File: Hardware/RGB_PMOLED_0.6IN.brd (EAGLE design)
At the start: 160 x 100 mm, 25 parts, among them Q1 310mA/60V/1.6Ω, U1 UG-6464TDDBG01-EXT, U2 AP3012, U3 3.3V, U4 TXB0104

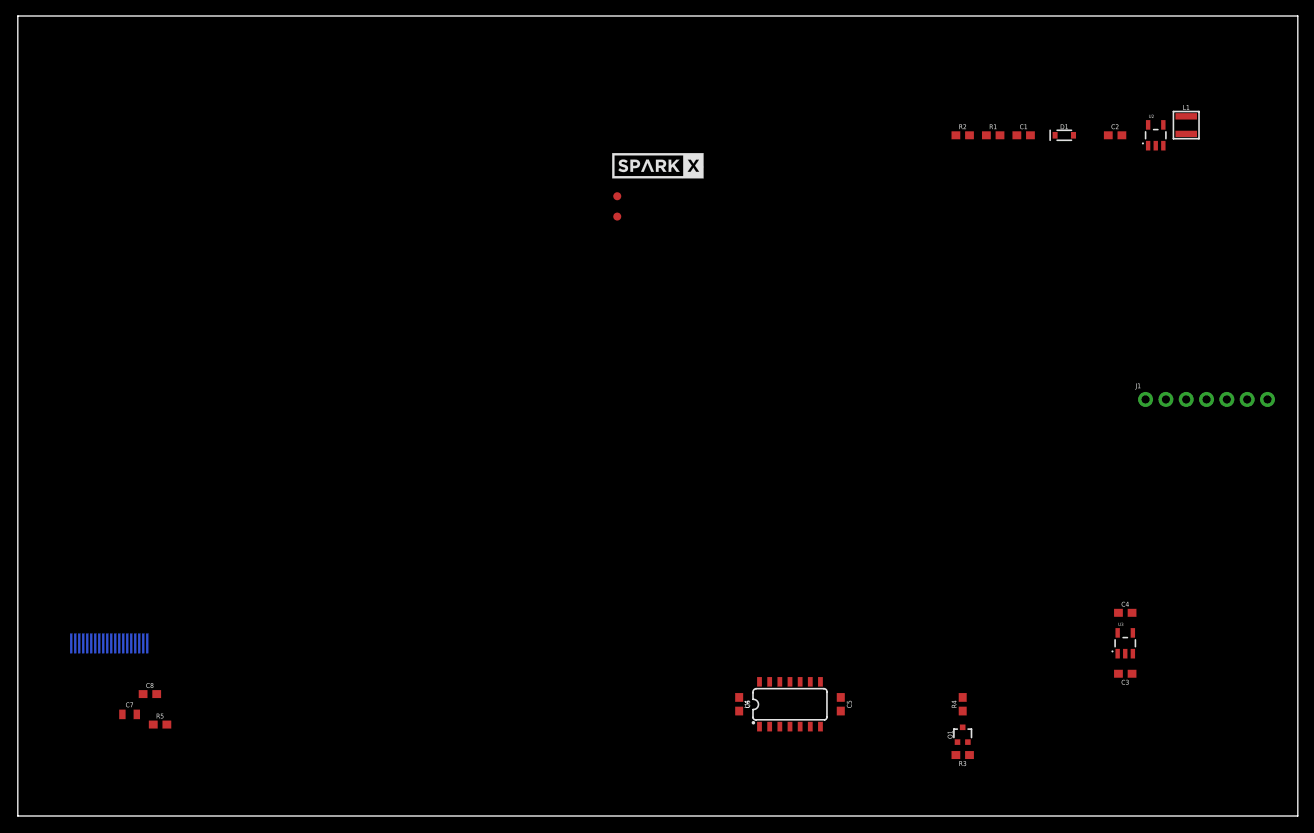
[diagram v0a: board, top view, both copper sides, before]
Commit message: First revision
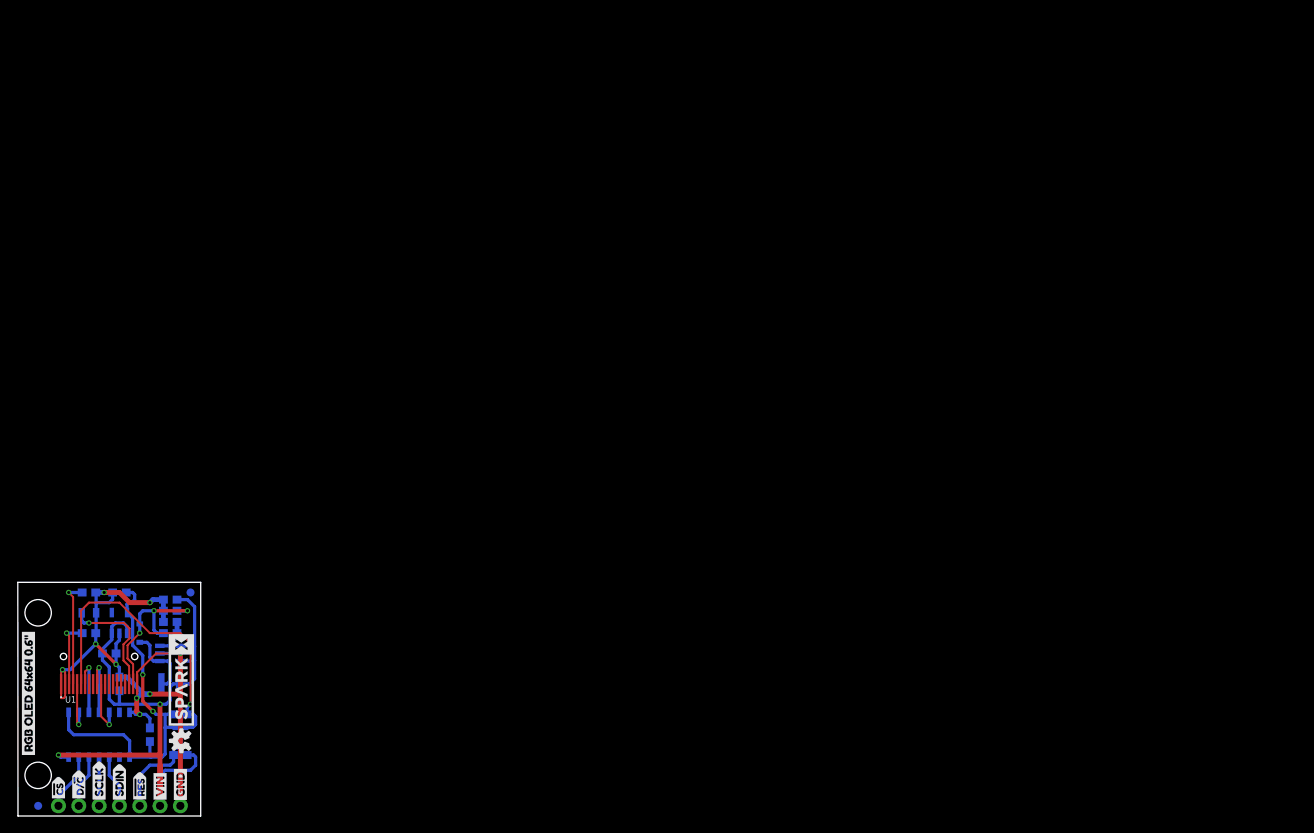
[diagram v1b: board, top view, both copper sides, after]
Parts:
- added H1, H2: STAND-OFF, SparkFun-Hardware:STAND-OFF
- added LOGO2, LOGO4: OSHW-LOGOS, SparkFun-Aesthetics:OSHW-LOGO-S
- added LOGO3: SPARKX-LOGO5, 1.81_Greyscale_OLED_Breakout:SPARKX-LARGE
- added U$1, U$2: (no value), buzzard_labels:VIN0
- added U$10, U$11: (no value), buzzard_labels:#RES2
- added U$12, U$13: (no value), buzzard_labels:#CS6
- added U$14, U$9: (no value), buzzard_labels:D##C5
- added U$16: (no value), buzzard_labels:RGB_OLED_64X64_0#6#7
- added U$3, U$4: (no value), buzzard_labels:SDIN3
- added U$5, U$6: (no value), buzzard_labels:SCLK4
- added U$7, U$8: (no value), buzzard_labels:GND1
- C7: value 2.2uF/25V -> 2.2uF
- U1: value UG-6464TDDBG01-EXT -> UG-6464TDDBG01-FLD; device RGB_OLED:UG-6464TDDBG01-EXTENDED -> RGB_OLED:UG-6464TDDBG01-FOLDED
- moved L1 144.9 mm to (19.1, 16.5), flipped to the bottom, turned to 90 degrees
- moved U2 139.2 mm to (19.1, 20.3), flipped to the bottom, turned to 90 degrees
- moved C2 132.2 mm to (19.1, 25.7), flipped to the bottom
- moved D1 131.3 mm to (15.2, 22.9), flipped to the bottom, turned to 270 degrees
- moved J1 130.9 mm to (20.3, 1.27), flipped to the bottom
- moved C3 127.0 mm to (11.4, 20.3), flipped to the bottom
- moved FRAME1 126.7 mm to (34.3, -14.0), flipped to the bottom
- moved C4 125.8 mm to (12.7, 27.9), flipped to the bottom
- moved U3 125.8 mm to (12.7, 24.1), flipped to the bottom
- moved C1 121.4 mm to (19.1, 27.1), flipped to the bottom
- moved R1 120.2 mm to (19.1, 22.9), flipped to the bottom
- moved R2 116.2 mm to (19.1, 24.3), flipped to the bottom, turned to 180 degrees
- moved FD2 103.3 mm to (2.54, 1.27), flipped to the bottom
- moved LOGO1 100.3 mm to (2.54, 17.5), flipped to the bottom, turned to 90 degrees
- moved R4 98.0 mm to (20.3, 7.62), flipped to the bottom, turned to 180 degrees
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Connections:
- removed net !CS!: U4.5
- net !CS: now also U4.2
- net !CS!_HIGH: now also J1.7, U4.13; no longer J1.4, U4.10
- net D/!C!_HIGH: now also J1.6; no longer J1.5
- net GND: now also C7.2; no longer C7.1
- net N$5: now also C7.1; no longer C7.2
- net SCLK_HIGH: now also J1.5; no longer J1.6
- net SDIN: now also U4.5; no longer U4.2
- net SDIN_HIGH: now also J1.4, U4.10; no longer J1.7, U4.13
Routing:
- net GND: track 0.00 -> 93.0 mm, vias 0 -> 9
- net VIN: track 0.00 -> 86.0 mm, vias 0 -> 2
- net 3.3V: track 0.00 -> 46.5 mm, vias 0 -> 2
- net !RES: track 0.00 -> 38.0 mm, vias 0 -> 1
- net 12V: track 0.00 -> 22.4 mm, vias 0 -> 3
- net N$5: track 0.00 -> 14.9 mm, vias 0 -> 1
- net N$11: track 0.00 -> 13.4 mm, vias 0 -> 1
- net !RES!_HIGH: track 0.00 -> 11.8 mm
- net N$2: track 0.00 -> 9.20 mm
- net N$10: track 0.00 -> 8.44 mm, vias 0 -> 1
- net D/!C: track 0.00 -> 7.83 mm, vias 0 -> 1
- net SCLK: track 0.00 -> 7.74 mm, vias 0 -> 1
- net !CS!_HIGH: track 0.00 -> 7.14 mm
- net SDIN: track 0.00 -> 7.01 mm, vias 0 -> 1
- net !CS: track 0.00 -> 6.68 mm, vias 0 -> 1
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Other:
- board size 160 x 100 mm -> 22.9 x 29.2 mm
- board text added: "Owen Lyke"

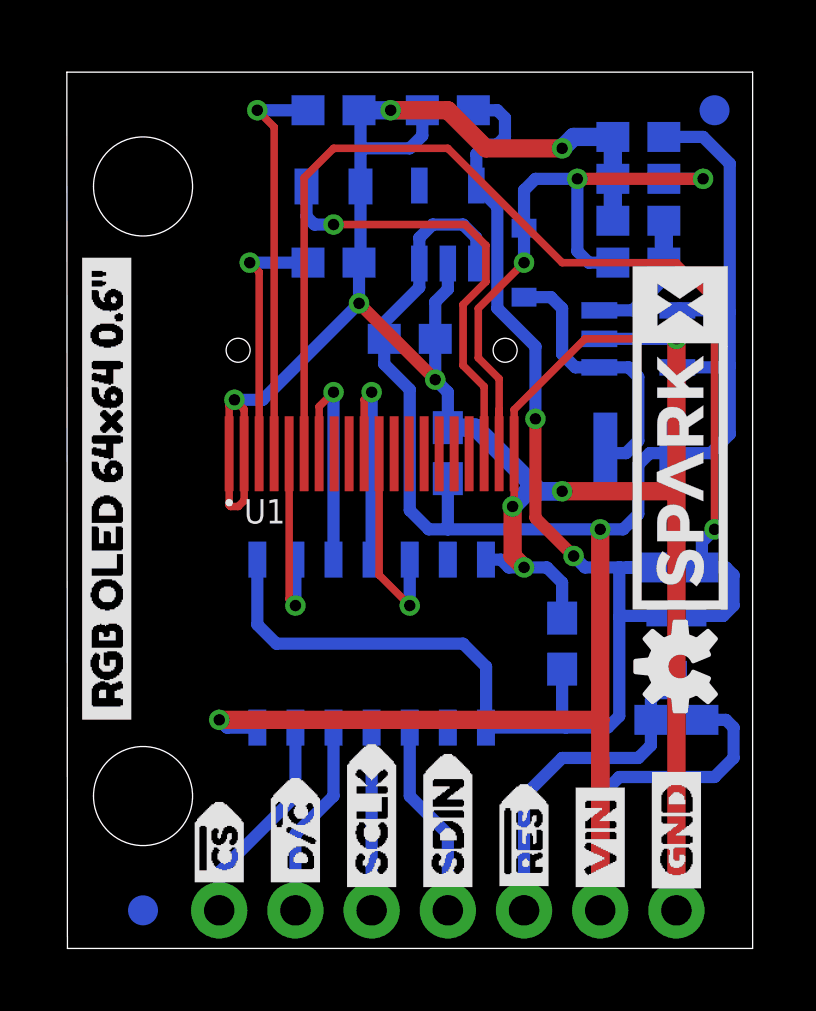
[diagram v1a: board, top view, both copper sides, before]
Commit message: Panelized and gerberified
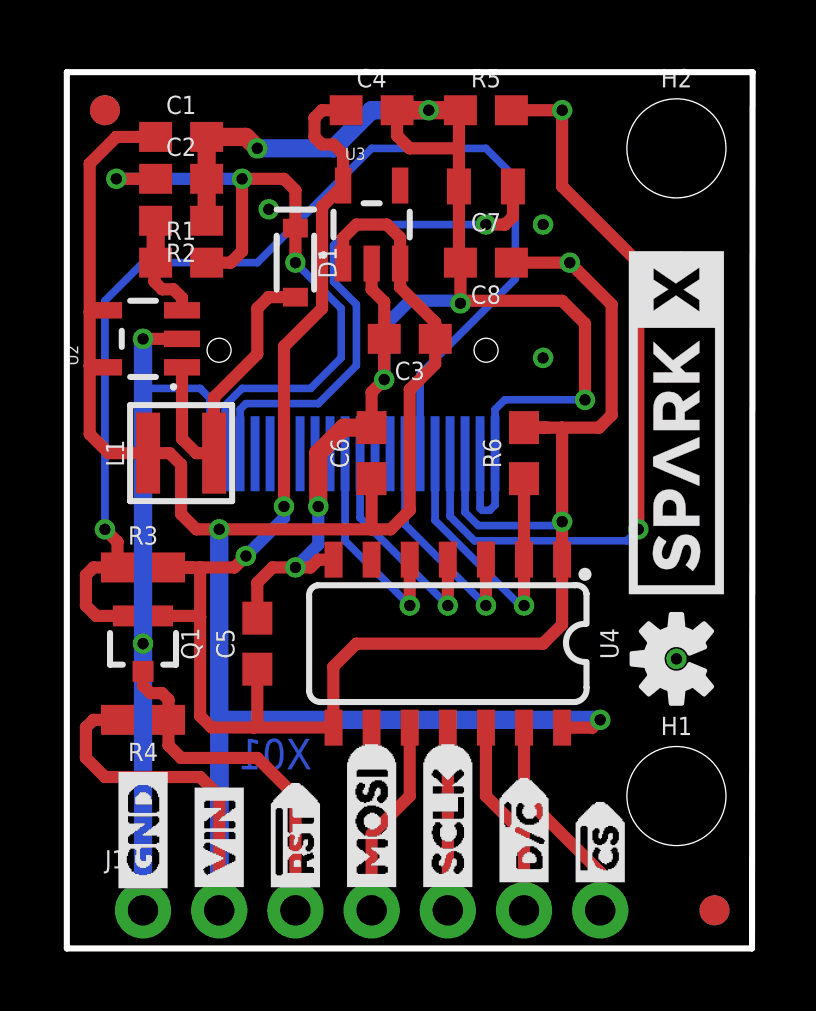
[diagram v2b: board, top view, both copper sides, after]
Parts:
- removed LOGO3: SPARKX-LOGO5, 1.81_Greyscale_OLED_Breakout:SPARKX-LARGE
- removed LOGO4: OSHW-LOGOS, SparkFun-Aesthetics:OSHW-LOGO-S
- added FD3, FD4: FIDUCIAL1X2, SparkFun-Aesthetics:FIDUCIAL-1X2
- added R6: 10k, SparkFun-Resistors:0603
- L1: device 1.81_Greyscale_OLED_Breakout:INDUCTOR_3X3 -> SparkFun-Coils:INDUCTOR_3X3
- U$10, U$11: device buzzard_labels:#RES2 -> buzzard_labels:#RST0
- U$3, U$4: device buzzard_labels:SDIN3 -> buzzard_labels:MOSI1
- U$5, U$6: device buzzard_labels:SCLK4 -> buzzard_labels:SCLK2
- U2: device 1.81_Greyscale_OLED_Breakout:SOT23-5 -> SparkFun-IC-Power:SOT23-5
- moved FRAME1 45.7 mm to (-11.4, -14.0), flipped to the top
- moved FD1 20.3 mm to (1.27, 27.9), flipped to the top
- moved U$16 20.2 mm to (21.5, 7.11), flipped to the bottom
- moved FD2 19.1 mm to (21.6, 1.27), flipped to the top
- moved H2 17.8 mm to (20.3, 26.7), flipped to the top
- moved H1 17.8 mm to (20.3, 5.08), flipped to the top
- moved J1 17.8 mm to (2.54, 1.27), flipped to the top
- moved LOGO1 17.8 mm to (20.3, 17.5), flipped to the top
- moved LOGO2 17.8 mm to (20.3, 9.65), flipped to the top
- moved Q1 17.8 mm to (2.54, 10.2), flipped to the top
- moved R3 17.8 mm to (2.54, 12.7), flipped to the top
- moved R4 17.8 mm to (2.54, 7.62), flipped to the top
- moved U$7 17.8 mm to (2.54, 1.52), flipped to the top
- moved U$8 17.8 mm to (2.54, 1.52), flipped to the bottom
- moved U2 16.5 mm to (2.54, 20.3), flipped to the top
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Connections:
- removed net N$10: C8.1, U1.18
- net !CS: now also R6.1
- net 3.3V: now also C8.1, R6.2, U1.18
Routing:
- net 3.3V: track 46.5 -> 67.8 mm, vias 2 -> 4
- net N$11: track 13.4 -> 25.6 mm, vias 1 -> 2
- net GND: track 93.0 -> 83.7 mm, vias 9 -> 12
- net N$10: track 8.44 -> 0.00 mm, vias 1 -> 0
- net !CS: track 6.68 -> 10.6 mm
- net N$5: track 14.9 -> 17.7 mm
- net VIN: track 86.0 -> 83.4 mm
- net !RES: track 38.0 -> 39.3 mm
- net N$2: track 9.20 -> 10.5 mm
- net 12V: track 22.4 -> 23.5 mm
- net N$3: track 4.53 -> 3.61 mm
- added copper zone on layer 1, net GND
- added copper zone on layer 16, net GND
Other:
- outline, holes or cut-outs redrawn
- board text added: "X01"
